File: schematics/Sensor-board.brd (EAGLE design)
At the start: 25 x 64 mm, 5 parts, among them U1 TSL2561, U2 TSL2561, U3 TSL2561, U4 MM74HC08M

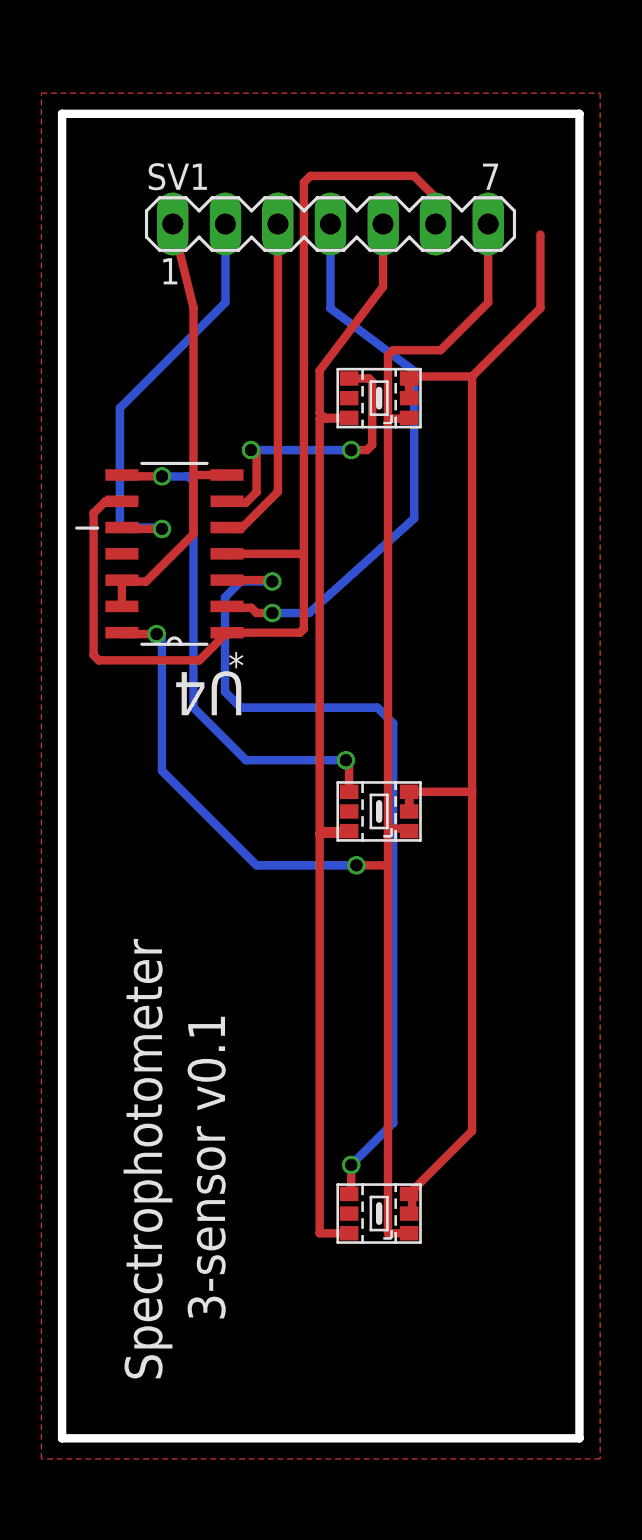
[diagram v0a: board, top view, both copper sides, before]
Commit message: Reworked some schematics
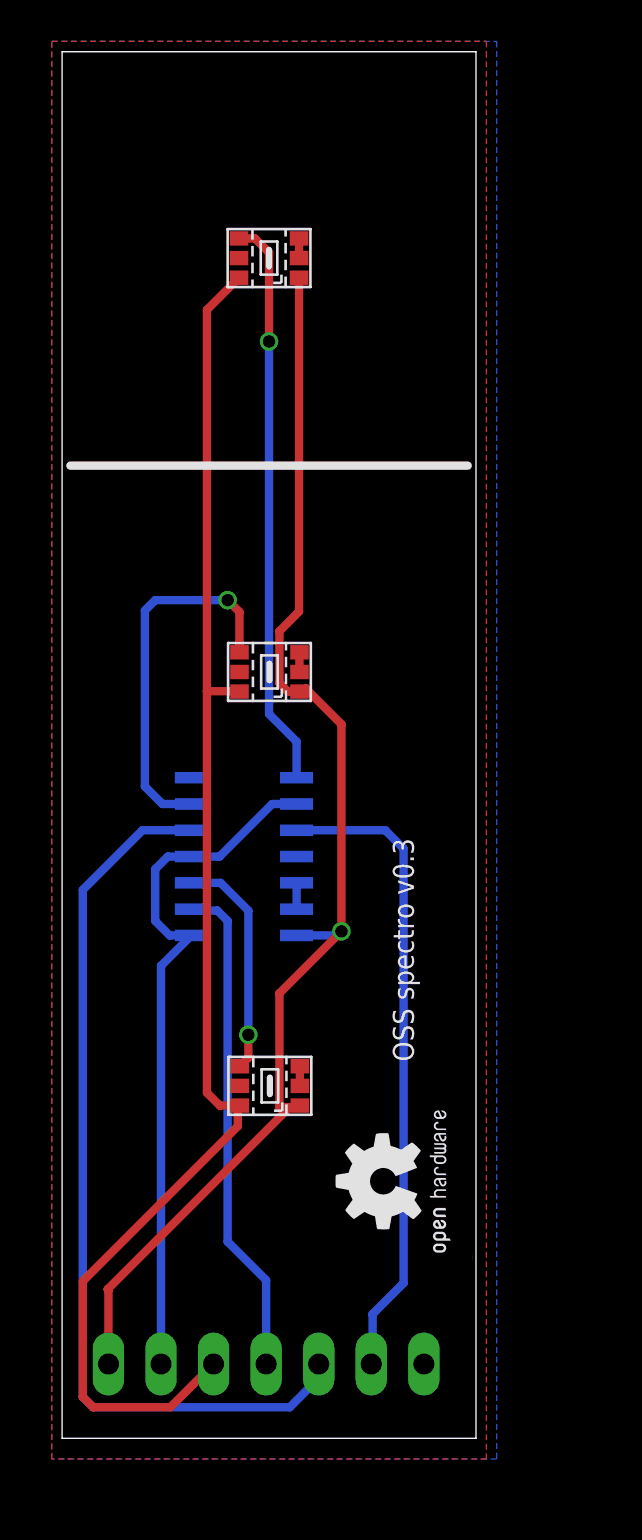
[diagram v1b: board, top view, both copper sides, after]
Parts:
- added U$1: (no value), bfl:OSHW2
- moved SV1 55.2 mm to (9.86, 3.59), flipped to the bottom
- moved U3 27.3 mm to (10.0, 57.0)
- moved U4 15.0 mm to (8.79, 28.1), flipped to the bottom
- moved U2 14.3 mm to (10.0, 37.0)
- moved U1 8.12 mm to (10.0, 17.0)
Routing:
- net GND: track 84.0 -> 4.12 mm
- net N$4: track 41.8 -> 11.0 mm, vias 2 -> 1
- net N$7: track 16.2 -> 43.8 mm
- net SCL: track 53.0 -> 34.0 mm
- net VCC: track 76.5 -> 63.0 mm, vias 2 -> 1
- net SDA: track 56.9 -> 68.1 mm
- net N$8: track 20.7 -> 31.1 mm, vias 1 -> 0
- net N$1: track 14.2 -> 18.1 mm, vias 2 -> 1
- net N$2: track 24.5 -> 27.7 mm, vias 2 -> 1
- net N$6: track 27.2 -> 24.2 mm, vias 1 -> 0
- added copper zone on layer 16, net GND
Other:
- board size 25 x 64 mm -> 20 x 67 mm
- board text added: "OSS spectro v0.3"
- board text removed: "3-sensor v0.1"
- board text removed: "Spectrophotometer"
